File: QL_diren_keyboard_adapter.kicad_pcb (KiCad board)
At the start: 2 copper layers, 47 x 54.6 mm, 12 parts, among them J1 Conn_01x20_Pin, J2 Conn_01x20_Pin, J3 Conn_01x05, J4 Conn_01x02, J5 Conn_01x03, U1 8749, U2 PIC16C5X, Y1 20Mhz

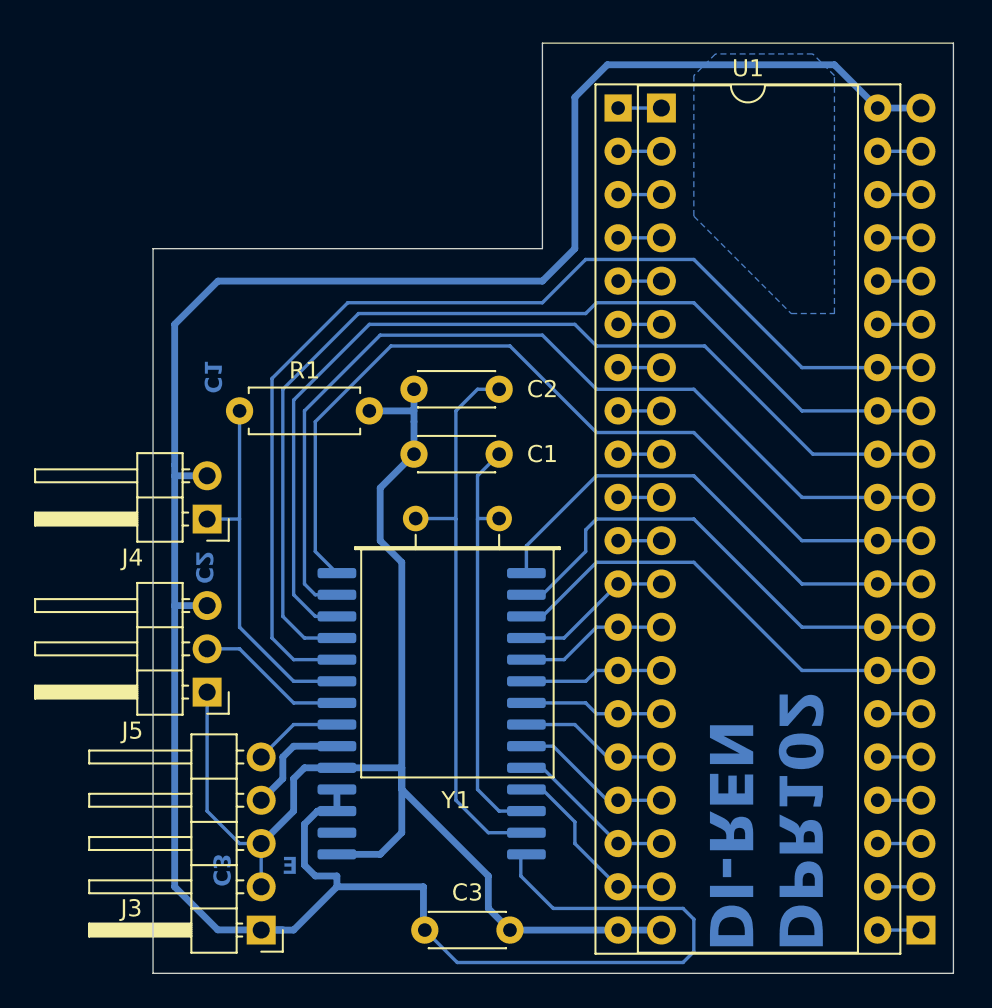
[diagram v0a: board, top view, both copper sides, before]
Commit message: updated
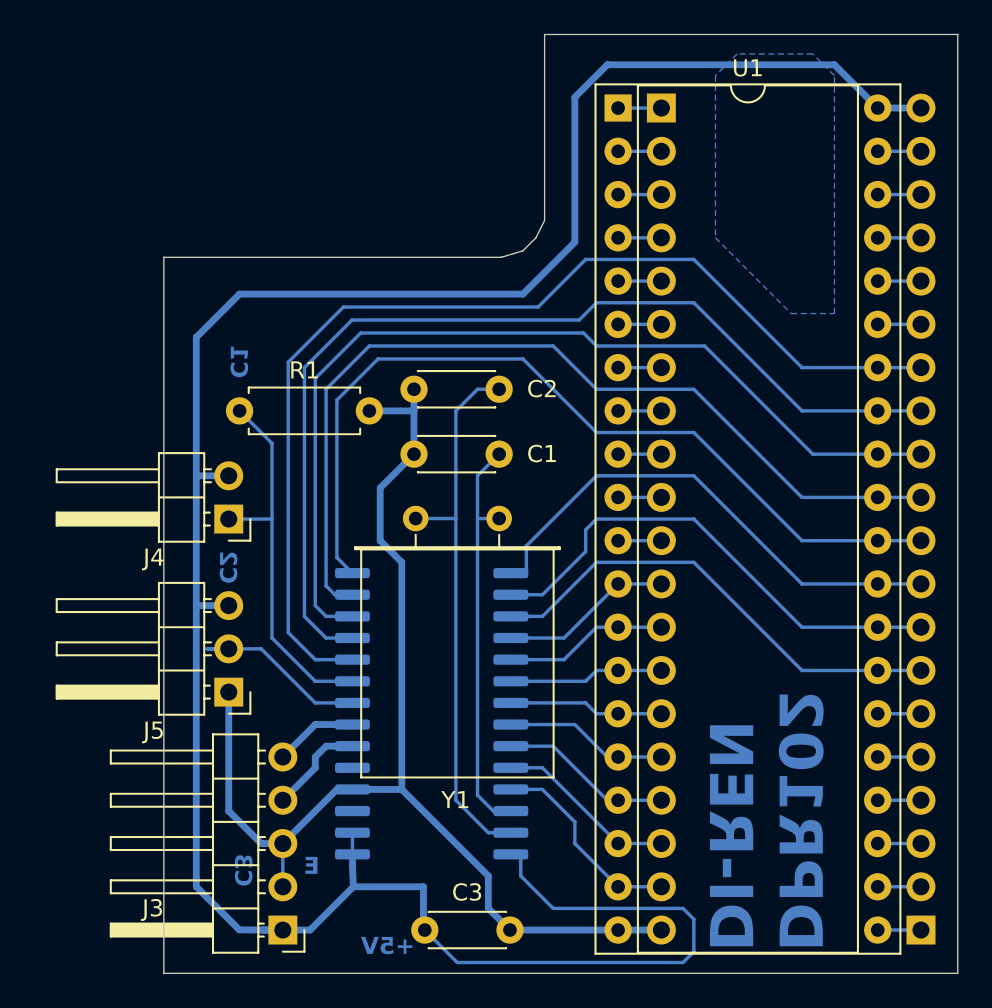
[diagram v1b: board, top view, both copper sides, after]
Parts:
- C1, C2: value 27p -> 15p
- J1, J2: value Conn_01x20_Pin -> Turned Pins 1x20
- J4: value Conn_01x02 -> JUMPER PINS x02
- J5: value Conn_01x03 -> JUMPER PINS x03
- U1: value 8749 -> SOCKET 40 PIN
- U2: value PIC16C5X -> PIC16C57-HS/SO; footprint Package_SO:SOP-28_8.4x18.16mm_P1.27mm -> Package_SO:SOIC-28W_7.5x17.9mm_P1.27mm
- Y1: value 20Mhz -> 10Mhz
- moved J3 1.27 mm to (81.9, 111.8)
- moved J4 1.27 mm to (78.7, 87.6)
- moved J5 1.27 mm to (78.7, 97.8)
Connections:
- U2 pad 1: GND -> +5V
- U2 pad 2: unconnected-(U2-TOCKI-Pad2) -> +5V
- U2 pad 3: +5V -> unconnected-(U2-NC_1-Pad3)
- U2 pad 4: +5V -> GND
- U2 pad 5: GND -> unconnected-(U2-NC_2-Pad5)
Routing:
- net GND: track 79.4 -> 70.3 mm
- net +5V: track 153.6 -> 145.5 mm
- net Net-(J5-Pin_2): track 8.28 -> 11.8 mm
- net /KBO01: track 27.4 -> 29.3 mm
- net /KBO00: track 26.2 -> 28.0 mm
- net /KBI07: track 10.1 -> 11.9 mm
- net /KBI06: track 8.83 -> 10.7 mm
- net /KBI05: track 7.67 -> 9.52 mm
- net /KBI00: track 8.30 -> 10.2 mm
- net /KBI04: track 7.14 -> 8.99 mm
- net /KBI03: track 7.25 -> 9.10 mm
- net /KBI02: track 7.25 -> 9.10 mm
- net /KBI01: track 7.77 -> 9.63 mm
- net /KBO05: track 56.3 -> 54.5 mm
- net /KBO06: track 59.2 -> 57.4 mm
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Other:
- board size 47 x 54.6 mm -> 46.6 x 55.1 mm
- board text added: "+5V"
